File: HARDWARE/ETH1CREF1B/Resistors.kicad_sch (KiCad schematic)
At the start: 56 parts, among them K201 9012, K202 9012, K203 9012, K204 9012, K205 9012, K206 9012, K207 9012, K208 9012, K209 9012, K210 9012, K211 9012, K212 9012, K213 9012, K214 9012, K215 9012, K216 9012, K217 9012, K218 9012, K219 9012, K220 9012

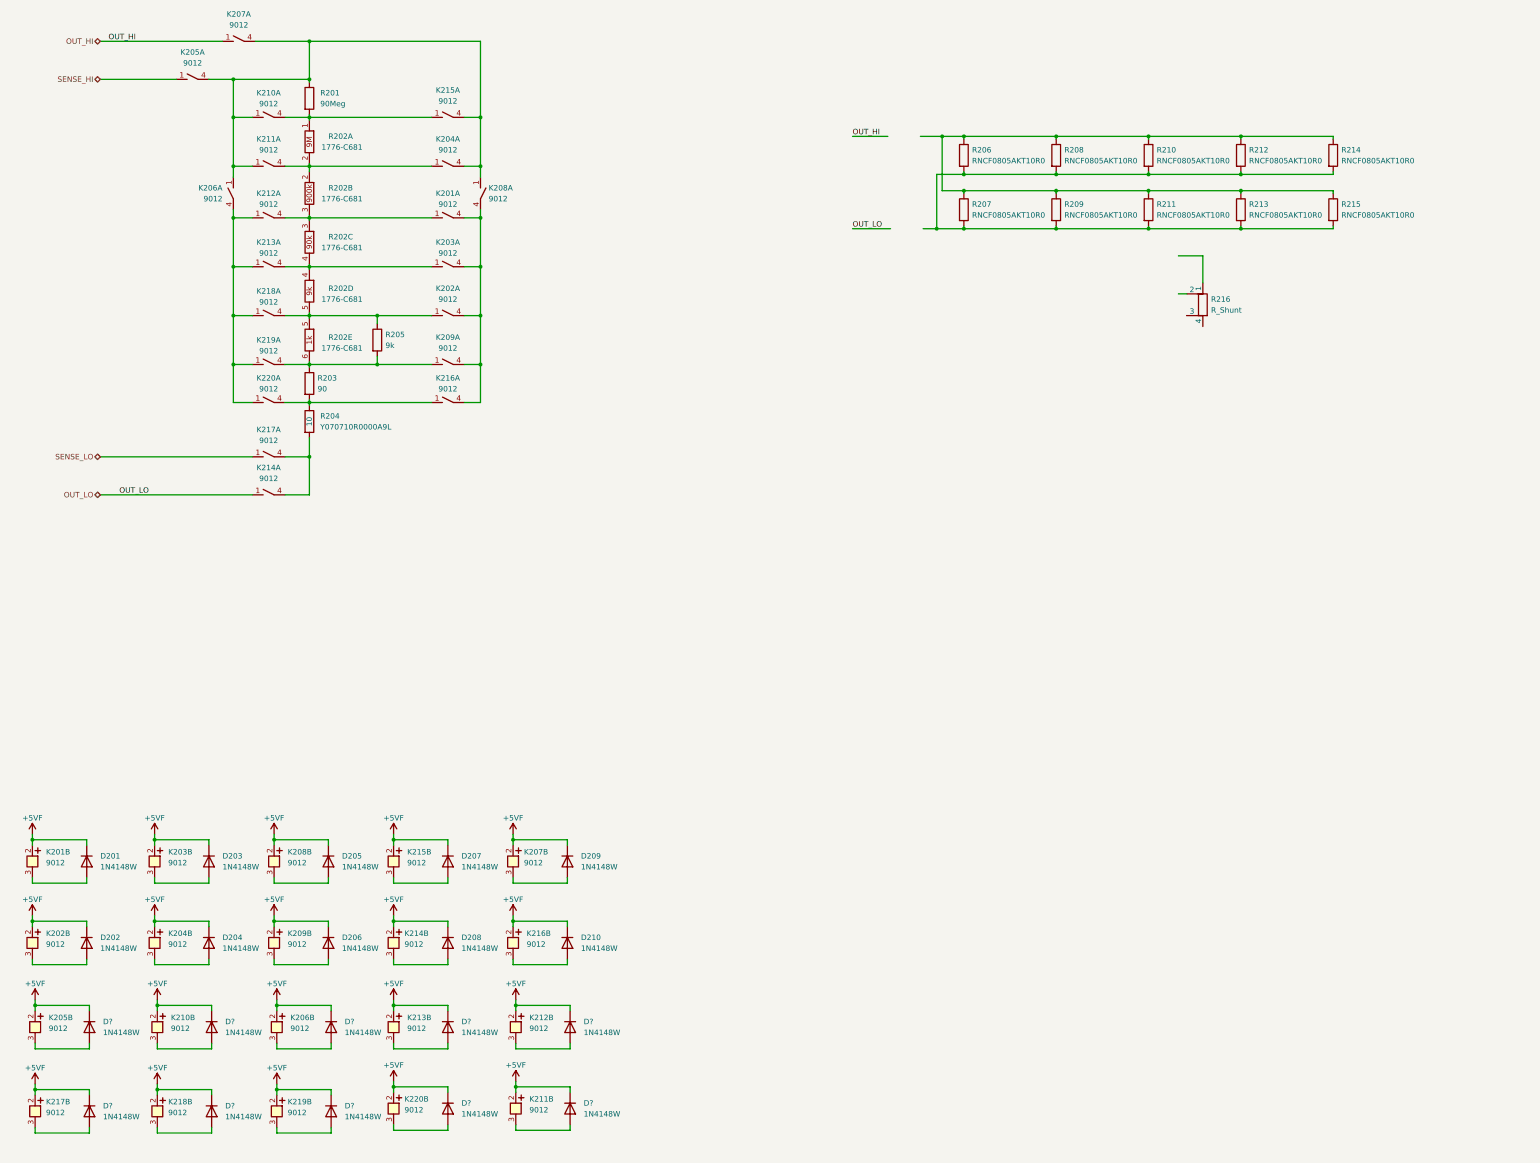
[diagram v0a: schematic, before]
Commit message: Hardware
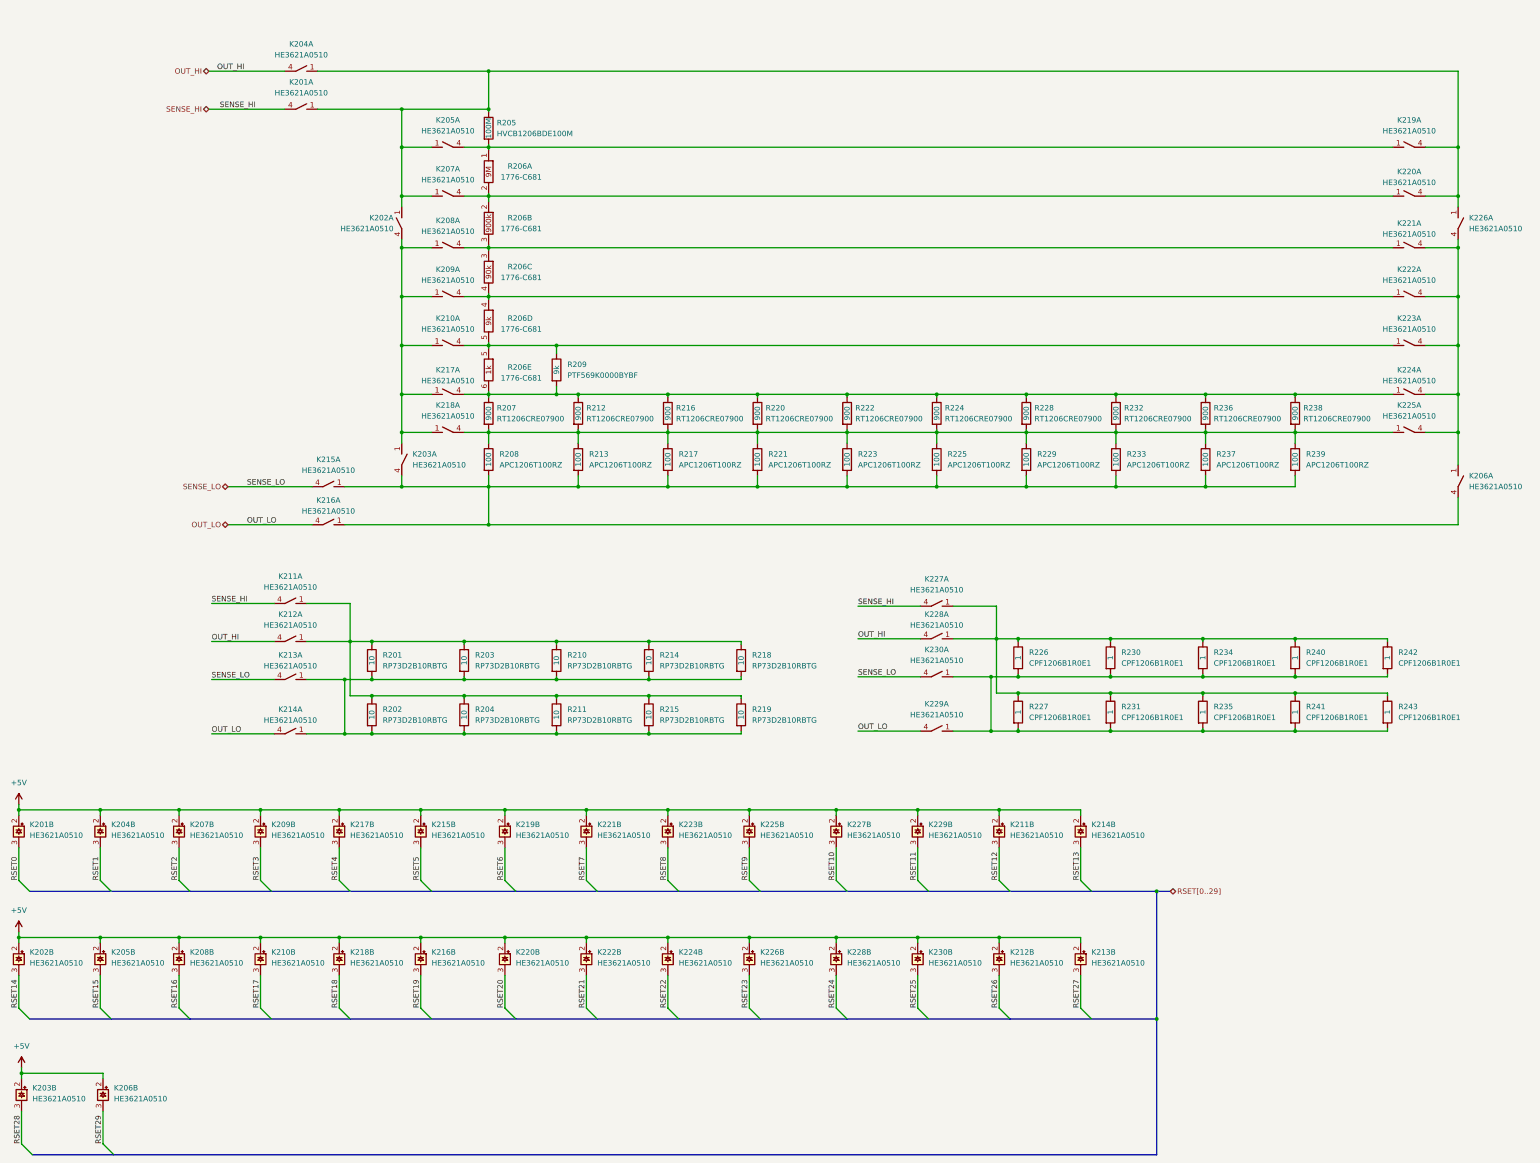
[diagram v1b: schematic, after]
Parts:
- removed D201, D202, D203, D204, D205, D206, D207, D208, D209, D210, D? (x10): 1N4148W, Diode_SMD:D_SOD-123, symbol Diode:1N4148W
- removed K201, K202, K203, K204, K205, K206, K207, K208, K209, K210, K211, K212, K213, K214, K215, K216, K217, K218, K219, K220: 9012, symbol ETH1CREF1A:9012
- removed R207, R208, R209: RNCF0805AKT10R0, symbol Device:R
- removed R216: R_Shunt, symbol Device:R_Shunt
- added K201, K202, K203, K204, K205, K206, K207, K208, K209, K210, K211, K212, K213, K214, K215, K216, K217, K218, K219, K220, K221, K222, K223, K224, K225, K226, K227, K228, K229, K230: HE3621A0510, ETH1CREF1B:HE360_x-5050462-8, symbol ETH1CREF1B:HE3621A0510
- added R202, R203, R204, R218, R219: RP73D2B10RBTG, Resistor_SMD:R_1206_3216Metric_Pad1.30x1.75mm_HandSolder, symbol Device:R
- added R216, R220, R222, R224, R228, R232, R236, R238: RT1206CRE07900, Resistor_SMD:R_1206_3216Metric_Pad1.30x1.75mm_HandSolder, symbol Device:R
- added R217, R221, R223, R225, R229, R233, R237, R239: APC1206T100RZ, Resistor_SMD:R_1206_3216Metric_Pad1.30x1.75mm_HandSolder, symbol Device:R
- added R226, R227, R230, R231, R234, R235, R240, R241, R242, R243: CPF1206B1R0E1, Resistor_SMD:R_1206_3216Metric_Pad1.30x1.75mm_HandSolder, symbol Device:R
- R201: renamed from R206; value RNCF0805AKT10R0 -> RP73D2B10RBTG; footprint (none) -> Resistor_SMD:R_1206_3216Metric_Pad1.30x1.75mm_HandSolder; User info (none) -> 10
- R205: renamed from R201; value 90Meg -> HVCB1206BDE100M; footprint (none) -> Resistor_SMD:R_1206_3216Metric_Pad1.30x1.75mm_HandSolder; User info (none) -> 100M
- R206: renamed from R202; footprint (none) -> ETH1CREF1B:1776-C681
- R207: renamed from R203; value 90 -> RT1206CRE07900; footprint (none) -> Resistor_SMD:R_1206_3216Metric_Pad1.30x1.75mm_HandSolder; Use info (none) -> 900
- R208: renamed from R204; value Y070710R0000A9L -> APC1206T100RZ; footprint (none) -> Resistor_SMD:R_1206_3216Metric_Pad1.30x1.75mm_HandSolder; User info 10 -> 100
- R209: renamed from R205; value 9k -> PTF569K0000BYBF; footprint (none) -> Resistor_THT:R_Axial_DIN0207_L6.3mm_D2.5mm_P15.24mm_Horizontal; User info (none) -> 9k
- R210, R211, R214, R215: value RNCF0805AKT10R0 -> RP73D2B10RBTG; footprint (none) -> Resistor_SMD:R_1206_3216Metric_Pad1.30x1.75mm_HandSolder; User info (none) -> 10
- R212: value RNCF0805AKT10R0 -> RT1206CRE07900; footprint (none) -> Resistor_SMD:R_1206_3216Metric_Pad1.30x1.75mm_HandSolder; Use info (none) -> 900
- R213: value RNCF0805AKT10R0 -> APC1206T100RZ; footprint (none) -> Resistor_SMD:R_1206_3216Metric_Pad1.30x1.75mm_HandSolder; User info (none) -> 100
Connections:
- net OUT_HI: now also K204.4, K212.4, K228.4
- net OUT_LO: now also K214.4, K216.4, K229.4
- net SENSE_HI: now also K201.4, K211.4, K227.4
- net SENSE_LO: now also K213.4, K215.4, K230.4
- net at R206.4, R206.4: now also K209.4, K222.1
- net at R206.5, R206.5, R209.1: now also K210.4, K223.1
- net at R201.1, R210.1, R211.1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: now also K211.1, K212.1, R202.1, R203.1, R204.1, R218.1, R219.1; no longer R212.1, R213.1
- net at R201.2, R210.2, R211.2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: now also K213.1, K214.1, R202.2, R203.2, R204.2, R218.2, R219.2; no longer R212.2, R213.2
- net at R208.2: now also R213.2, K203.4, K206.4, K215.1, K216.1, R217.2, R221.2, R223.2, R225.2, R229.2, R233.2, R237.2, R239.2
- net at R207.2, R208.1: now also R212.2, R213.1, K218.4, K225.1, R216.2, R217.1, R220.2, R221.1, R222.2, R223.1, R224.2, R225.1, R228.2, R229.1, R232.2, R233.1, R236.2, R237.1, R238.2, R239.1
- net at R205.1: now also K201.1, K202.1, K204.1, K205.1, K207.1, K219.4, K220.4, K226.1
- net at R206.6, R207.1, R209.2: now also R212.1, K217.4, K224.1, R216.1, R220.1, R222.1, R224.1, R228.1, R232.1, R236.1, R238.1
- net at R205.2, R206.1: now also K205.4, K219.1
- net at R206.2, R206.2: now also K207.4, K220.1
- net at R206.3, R206.3: now also K208.4, K221.1
- new net: K206.1, K221.4, K222.4, K223.4, K224.4, K225.4, K226.4
- new net: K227.1, K228.1, R226.1, R227.1, R230.1, R231.1, R234.1, R235.1, R240.1, R241.1, R242.1, R243.1
- new net: K229.1, K230.1, R226.2, R227.2, R230.2, R231.2, R234.2, R235.2, R240.2, R241.2, R242.2, R243.2
- new net: K202.4, K203.1, K208.1, K209.1, K210.1, K217.1, K218.1
- new net +5V: K201.2, K202.2, K203.2, K204.2, K205.2, K206.2, K207.2, K208.2, K209.2, K210.2, K211.2, K212.2, K213.2, K214.2, K215.2, K216.2, K217.2, K218.2, K219.2, K220.2, K221.2, K222.2, K223.2, K224.2, K225.2, K226.2, K227.2, K228.2, K229.2, K230.2
- new net RSET0: K201.3
- new net RSET1: K204.3
- new net RSET10: K227.3
- new net RSET11: K229.3
- new net RSET12: K211.3
- new net RSET13: K214.3
- new net RSET14: K202.3
- new net RSET15: K205.3
- new net RSET16: K208.3
- new net RSET17: K210.3
- new net RSET18: K218.3
- new net RSET19: K216.3
- new net RSET2: K207.3
- new net RSET20: K220.3
- new net RSET21: K222.3
- new net RSET22: K224.3
- new net RSET23: K226.3
- new net RSET24: K228.3
- new net RSET25: K230.3
- new net RSET26: K212.3
- new net RSET27: K213.3
- new net RSET28: K203.3
- new net RSET29: K206.3
- new net RSET3: K209.3
- new net RSET4: K217.3
- new net RSET5: K215.3
- new net RSET6: K219.3
- new net RSET7: K221.3
- new net RSET8: K223.3
- new net RSET9: K225.3
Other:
- moved on the sheet: R201, R205, R206A, R206B, R206C, R206D, R206E, R207, R208, R209
